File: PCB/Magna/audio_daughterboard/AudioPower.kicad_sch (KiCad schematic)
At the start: 54 parts, among them U901 TLV76701DRVx, U902 TLV61046ADBVR, U903 TLV76701DRVx, U904 TLV76701DRVx

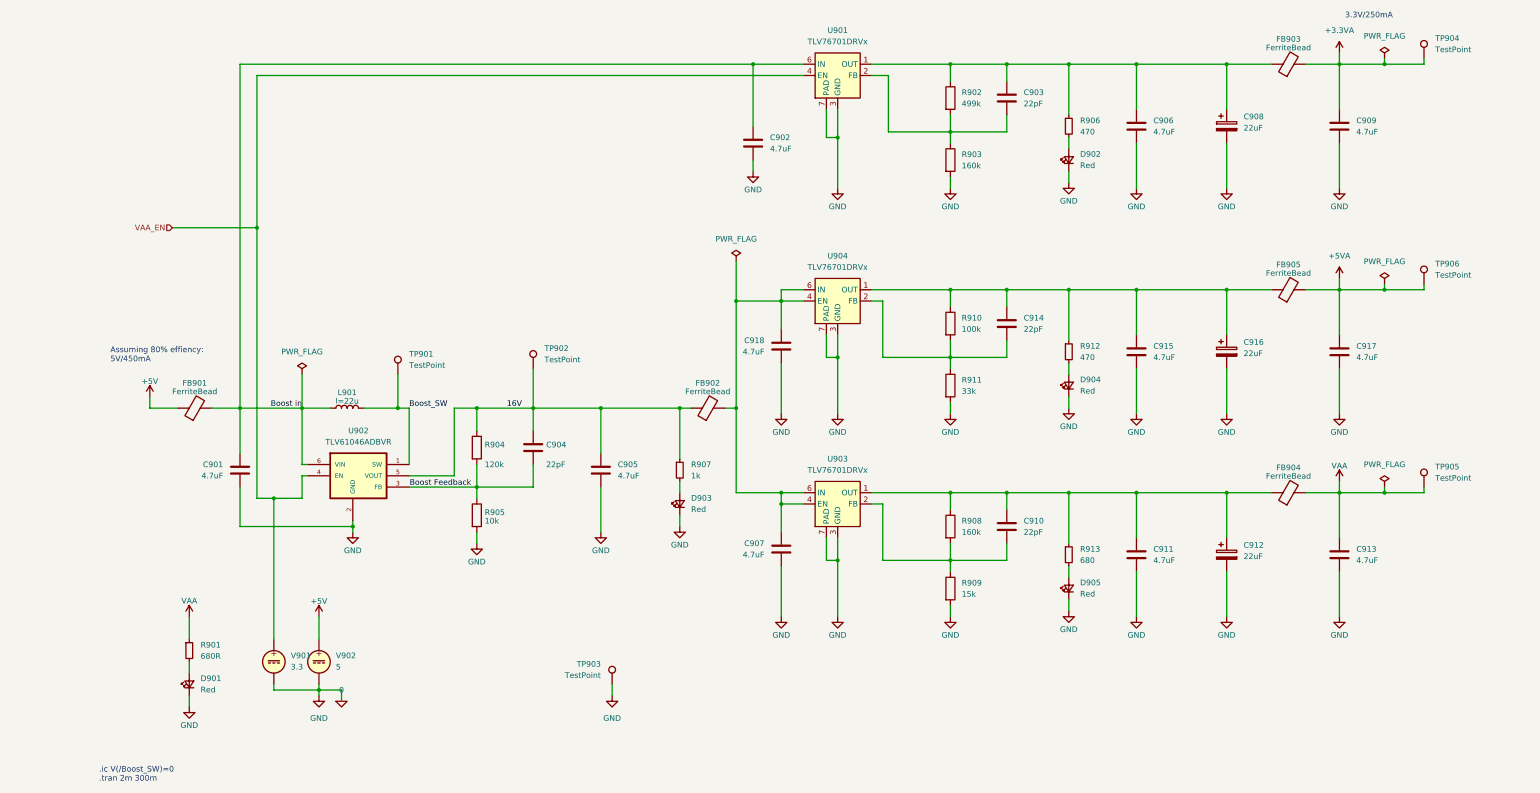
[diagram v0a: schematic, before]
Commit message: Some updates to PCB
Honestly I cannot remember whats changed
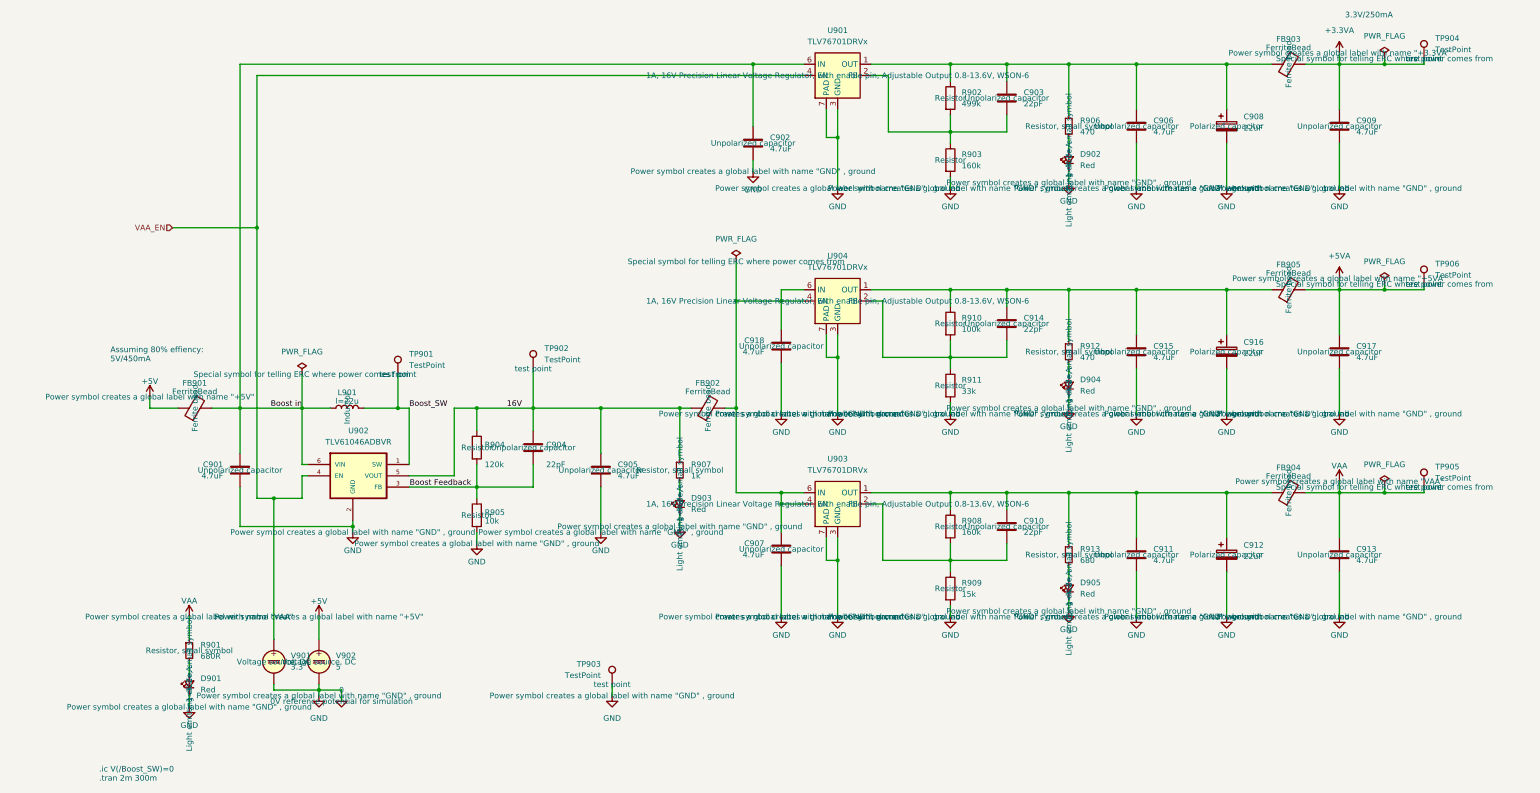
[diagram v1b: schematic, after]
